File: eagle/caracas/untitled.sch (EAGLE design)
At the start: 24 parts, among them IC1 4001N, Q1 IRLZ44Z, X1 22-23-2021, X2 22-23-2021, X3 22-23-2041, X4 22-23-2041, X5 22-23-2021, X6 22-23-2021

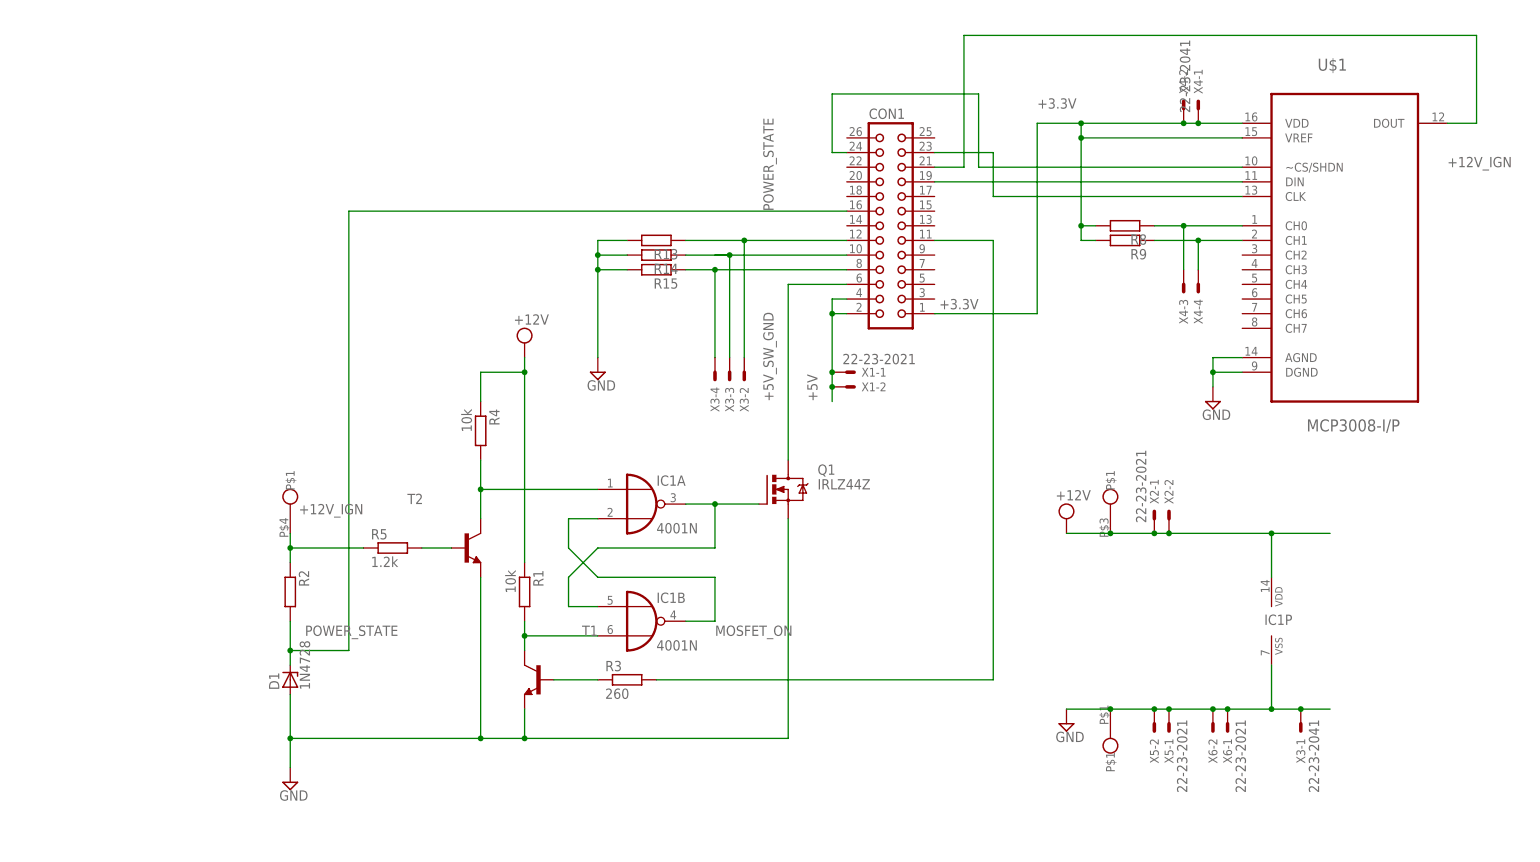
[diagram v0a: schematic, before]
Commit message: WIP schematics
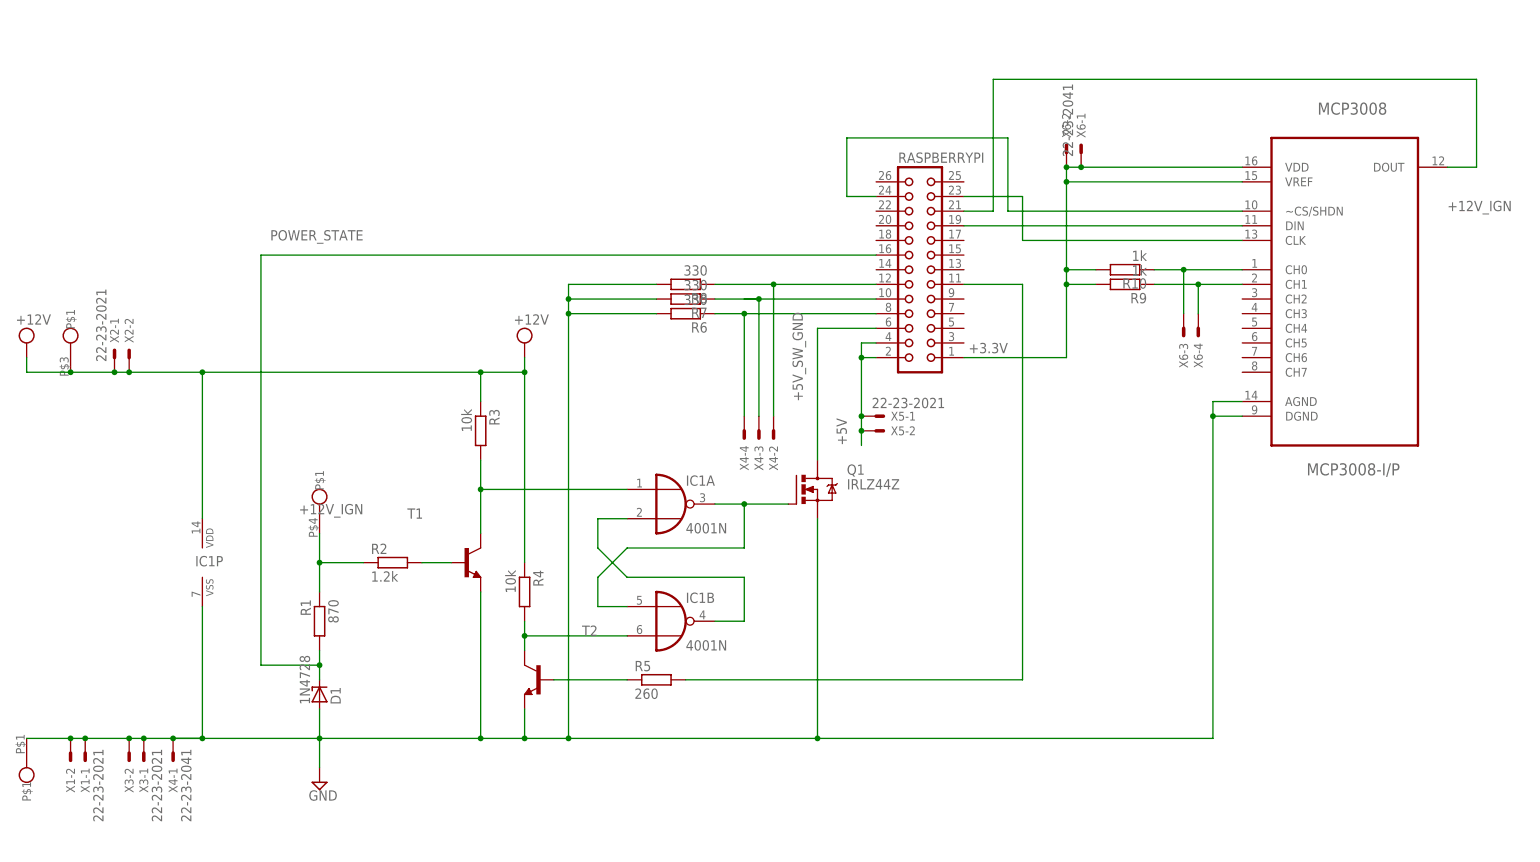
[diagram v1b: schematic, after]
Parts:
- removed CON1: (no value), con-harting:CON26
- removed R13, R14, R15: (no value), rcl:R-EU_0207/10
- removed U$2: MKDS3, caracas:MKDS3
- added MCP3008: MCP3008-I/P, mpc3008:MCP3008-I/P
- added R10: 1k, rcl:R-EU_0207/10
- added R6, R7: 330, rcl:R-EU_0207/10
- added RASPBERRYPI: (no value), con-harting:CON26
- R1: value 10k -> 870
- R2: value (none) -> 1.2k
- R3: value 260 -> 10k
- R5: value 1.2k -> 260
- R8: value (none) -> 330
- R9: value (none) -> 1k
- U$1: value MCP3008-I/P -> MKDS3; device mpc3008:MCP3008-I/P -> caracas:MKDS3
- X3: value 22-23-2041 -> 22-23-2021; device con-molex:22-23-2041 -> con-molex:22-23-2021
- X6: value 22-23-2021 -> 22-23-2041; device con-molex:22-23-2021 -> con-molex:22-23-2041
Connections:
- net +12V_IGN: now also R1.1, U$1G$4.P$1; no longer R5.1, U$2G$4.P$1
- net +3.3V: now also MCP3008.VDD, MCP3008.VREF, R10.2, RASPBERRYPI.1, X6-1.S, X6-2.S; no longer CON1.1, R8.2, U$1.VDD, U$1.VREF, X4-1.S, X4-2.S
- net +5V: now also RASPBERRYPI.2, RASPBERRYPI.4, X5-1.S, X5-2.S; no longer CON1.2, CON1.4, X1-1.S, X1-2.S
- net +5V_SW_GND: now also RASPBERRYPI.6; no longer CON1.6
- net ANA_0: now also MCP3008.CH0, R10.1, X6-3.S; no longer R8.1, U$1.CH0, X4-3.S
- net ANA_1: now also MCP3008.CH1, X6-4.S; no longer U$1.CH1, X4-4.S
- net GND: now also MCP3008.AGND, MCP3008.DGND, R6.2, R7.2, R8.2, U$1G$1.P$1, X1-1.S, X1-2.S, X3-2.S, X4-1.S; no longer R13.2, R14.2, R15.2, U$1.AGND, U$1.DGND, U$2G$1.P$1, X5-1.S, X5-2.S, X6-1.S, X6-2.S
- net N$10: now also R8.1, RASPBERRYPI.12, X4-2.S; no longer CON1.12, R13.1, X3-2.S
- net N$11: now also R3.2, T1.C; no longer R4.2, T2.C
- net N$12: now also R2.2, T1.B; no longer R5.2, T2.B
- net N$2: now also R4.2, T2.C; no longer R1.2, T1.C
- net N$3: now also MCP3008.CLK, RASPBERRYPI.23; no longer CON1.23, U$1.CLK
- net N$4: now also MCP3008.DOUT, RASPBERRYPI.21; no longer CON1.21, U$1.DOUT
- net N$5: now also MCP3008.DIN, RASPBERRYPI.19; no longer CON1.19, U$1.DIN
- net N$6: now also MCP3008.~CS/SHDN, RASPBERRYPI.24; no longer CON1.24, U$1.~CS/SHDN
- net N$7: now also R6.1, RASPBERRYPI.8, X4-4.S; no longer CON1.8, R15.1, X3-4.S
- net N$8: now also R7.1, RASPBERRYPI.10, X4-3.S; no longer CON1.10, R14.1, X3-3.S
- net N$9: now also R5.1, T2.B; no longer R3.1, T1.B
- net POWER_STATE: now also R1.2, RASPBERRYPI.16; no longer CON1.16, R2.2
- net RPI_RESET: now also R5.2, RASPBERRYPI.11; no longer CON1.11, R3.2
- net VCC: now also R3.1, U$1G$3.P$1; no longer R1.1, U$2G$3.P$1
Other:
- moved on the sheet: D1, IC1A, IC1B, IC1P, Q1, R1, R2, R3, R4, R5, R8, R9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
